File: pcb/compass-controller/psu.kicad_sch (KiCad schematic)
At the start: 16 parts, among them U301 TPS5430DDA

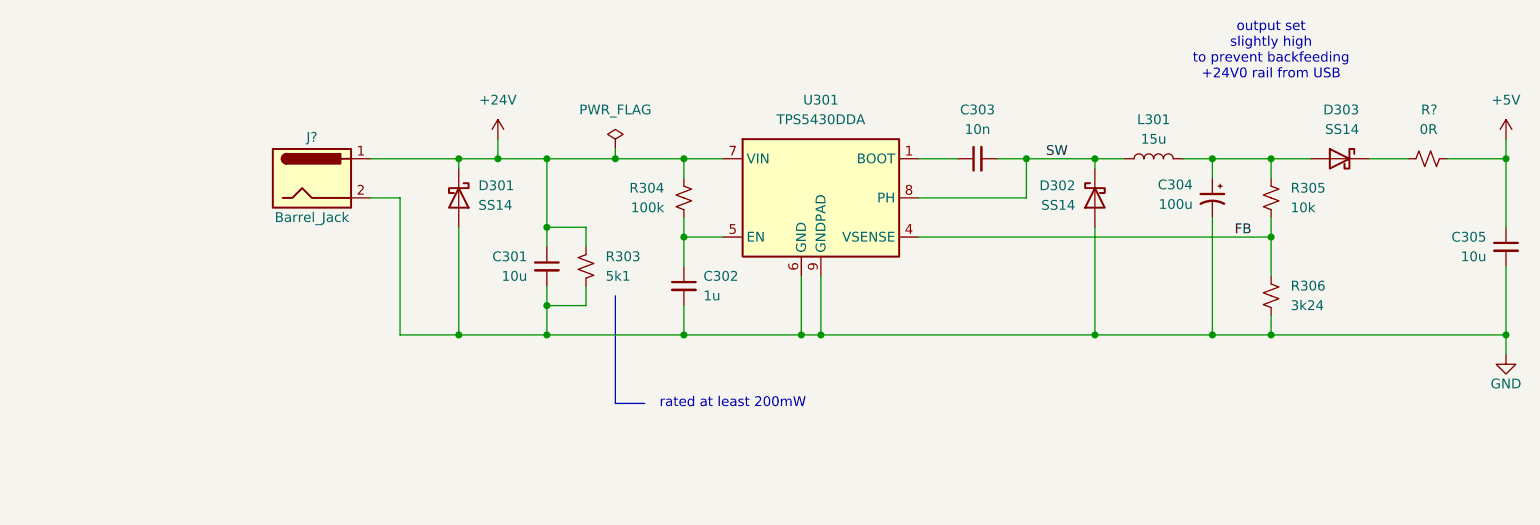
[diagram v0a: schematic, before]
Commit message: build platform
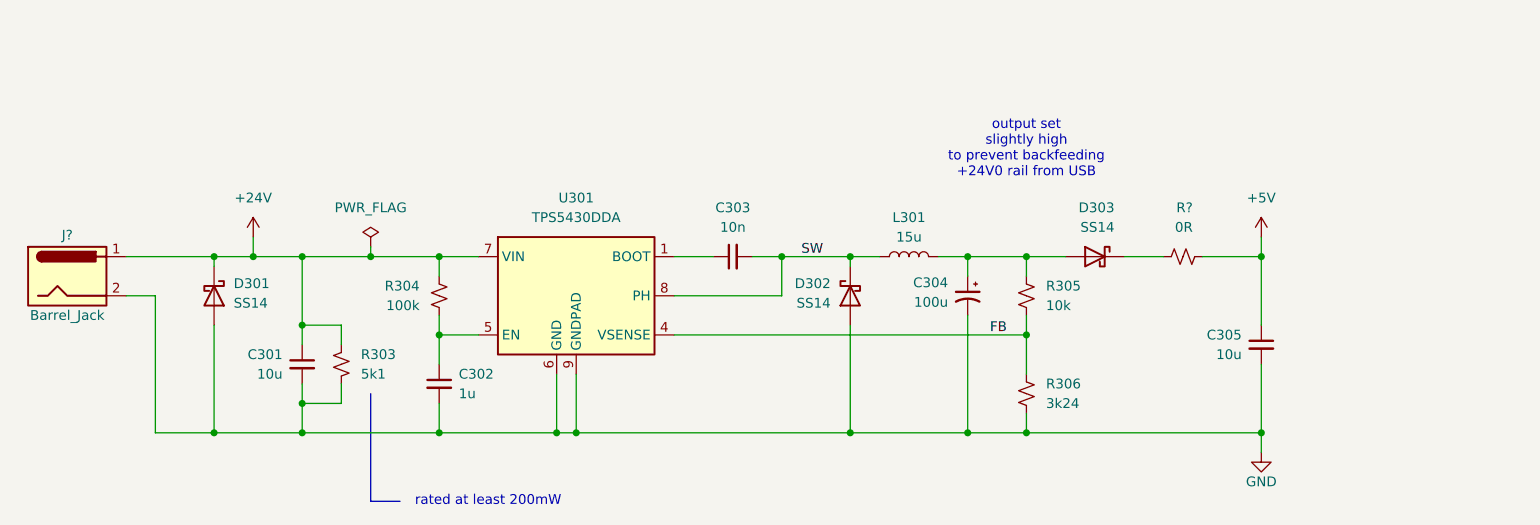
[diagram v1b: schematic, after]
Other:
- moved on the sheet: C301, C302, C303, C304, C305, D301, D302, D303, J?, L301, R303, R304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
